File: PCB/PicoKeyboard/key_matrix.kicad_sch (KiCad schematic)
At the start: 170 parts

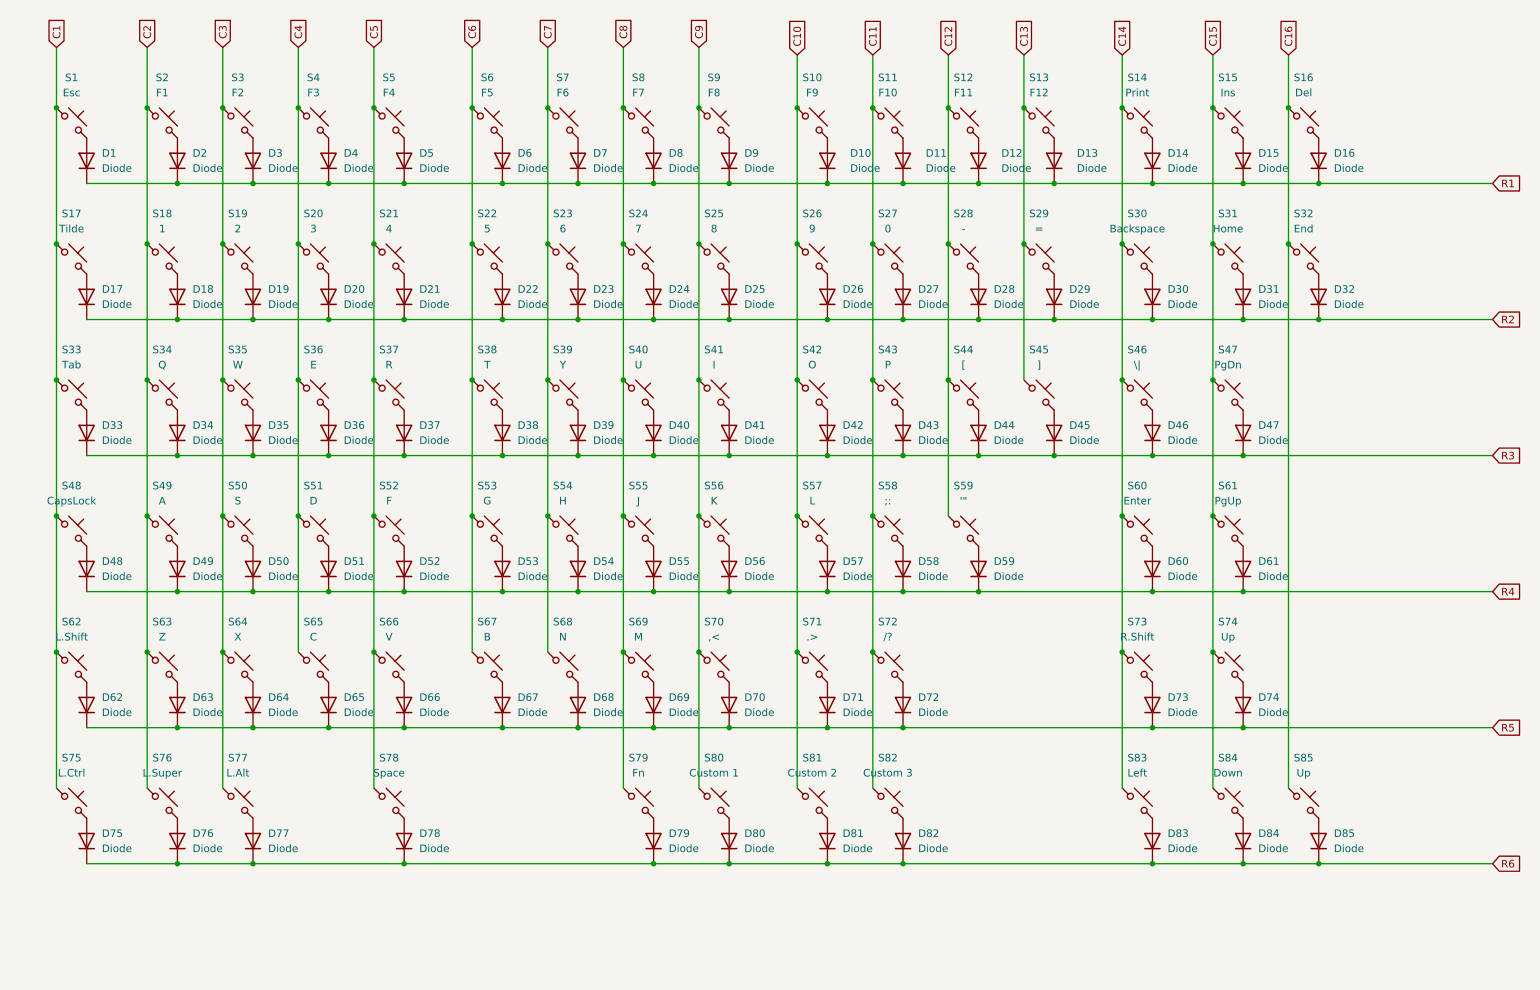
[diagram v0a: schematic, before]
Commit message: New layout
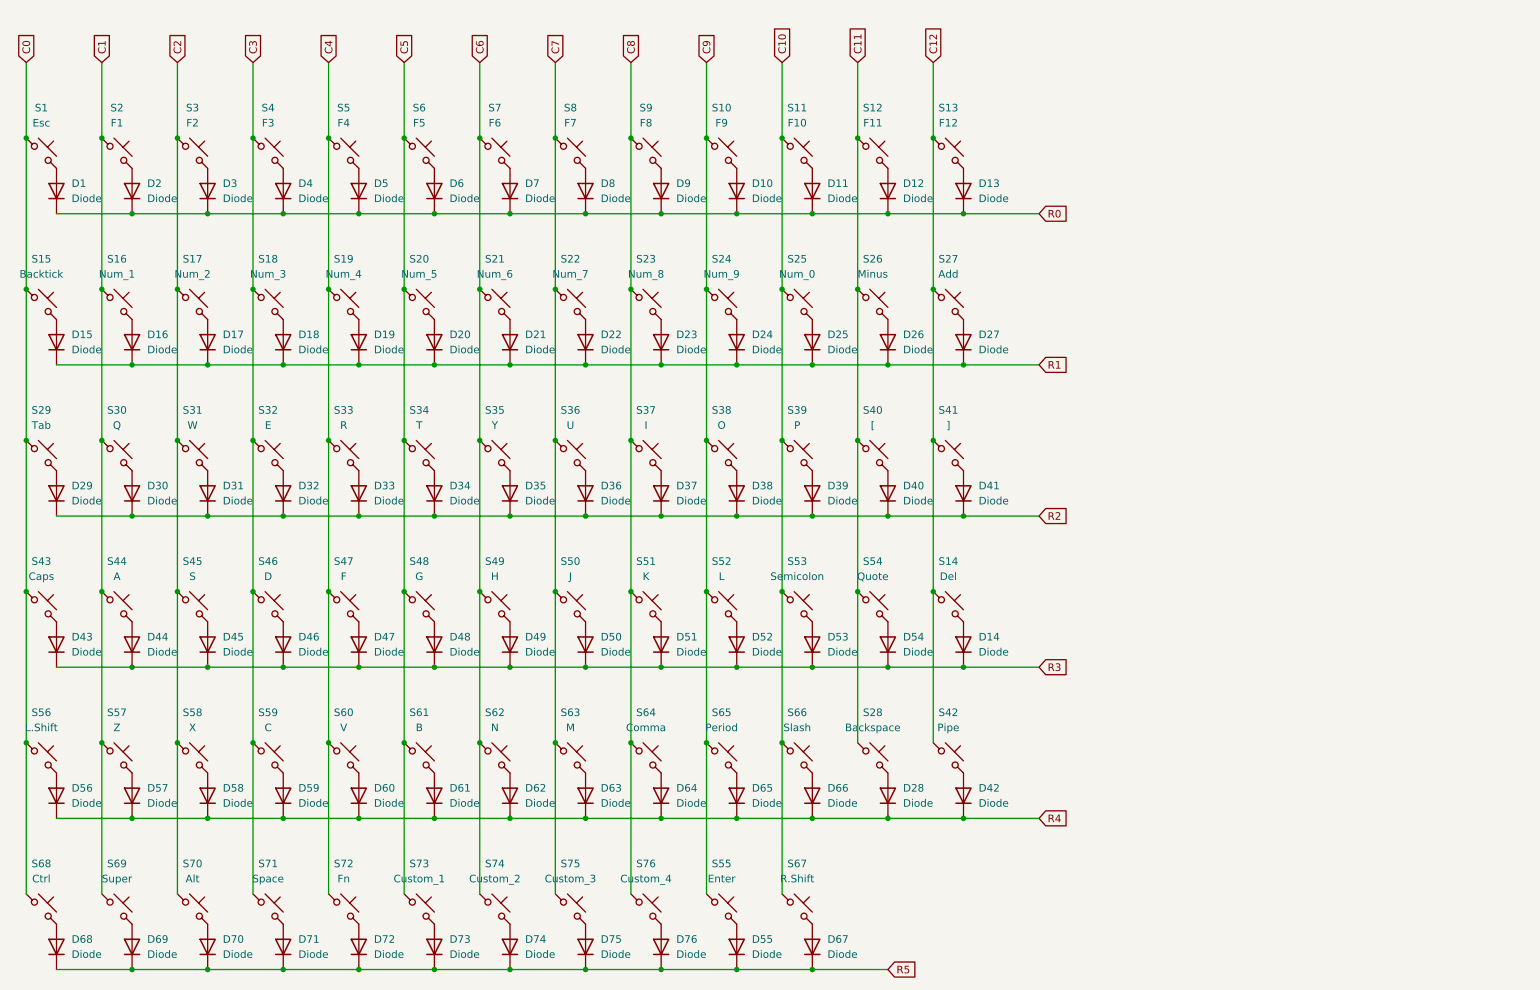
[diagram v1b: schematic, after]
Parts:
- removed D77, D78, D79, D80, D81, D82, D83, D84, D85: Diode, ScottoKeebs_Components:Diode_SOD-123, symbol ScottoKeebs:Placeholder_Diode
- removed S77: L.Alt, Button_Switch_Keyboard:SW_Cherry_MX_1.25u_PCB, symbol ScottoKeebs:Placeholder_Keyswitch
- removed S78: Space, Button_Switch_Keyboard:SW_Cherry_MX_6.25u_PCB, symbol ScottoKeebs:Placeholder_Keyswitch
- removed S79: Fn, Button_Switch_Keyboard:SW_Cherry_MX_1.00u_PCB, symbol ScottoKeebs:Placeholder_Keyswitch
- removed S80: Custom 1, Button_Switch_Keyboard:SW_Cherry_MX_1.00u_PCB, symbol ScottoKeebs:Placeholder_Keyswitch
- removed S81: Custom 2, Button_Switch_Keyboard:SW_Cherry_MX_1.00u_PCB, symbol ScottoKeebs:Placeholder_Keyswitch
- removed S82: Custom 3, Button_Switch_Keyboard:SW_Cherry_MX_1.00u_PCB, symbol ScottoKeebs:Placeholder_Keyswitch
- removed S83: Left, Button_Switch_Keyboard:SW_Cherry_MX_1.00u_PCB, symbol ScottoKeebs:Placeholder_Keyswitch
- removed S84: Down, Button_Switch_Keyboard:SW_Cherry_MX_1.00u_PCB, symbol ScottoKeebs:Placeholder_Keyswitch
- removed S85: Up, Button_Switch_Keyboard:SW_Cherry_MX_1.00u_PCB, symbol ScottoKeebs:Placeholder_Keyswitch
- S1, S10, S11, S12, S13, S2, S3, S4, S5, S6, S7, S8, S9: footprint Button_Switch_Keyboard:SW_Cherry_MX_1.00u_PCB -> ScottoKeebs_MX:MX_PCB_1.00u
- S14: value Print -> Del; footprint Button_Switch_Keyboard:SW_Cherry_MX_1.00u_PCB -> ScottoKeebs_MX:MX_PCB_1.00u
- S15: value Ins -> Backtick; footprint Button_Switch_Keyboard:SW_Cherry_MX_1.00u_PCB -> ScottoKeebs_MX:MX_PCB_1.00u
- S16: value Del -> Num_1; footprint Button_Switch_Keyboard:SW_Cherry_MX_1.00u_PCB -> ScottoKeebs_MX:MX_PCB_1.00u
- S17: value Tilde -> Num_2; footprint Button_Switch_Keyboard:SW_Cherry_MX_1.00u_PCB -> ScottoKeebs_MX:MX_PCB_1.00u
- S18: value 1 -> Num_3; footprint Button_Switch_Keyboard:SW_Cherry_MX_1.00u_PCB -> ScottoKeebs_MX:MX_PCB_1.00u
- S19: value 2 -> Num_4; footprint Button_Switch_Keyboard:SW_Cherry_MX_1.00u_PCB -> ScottoKeebs_MX:MX_PCB_1.00u
- S20: value 3 -> Num_5; footprint Button_Switch_Keyboard:SW_Cherry_MX_1.00u_PCB -> ScottoKeebs_MX:MX_PCB_1.00u
- S21: value 4 -> Num_6; footprint Button_Switch_Keyboard:SW_Cherry_MX_1.00u_PCB -> ScottoKeebs_MX:MX_PCB_1.00u
- S22: value 5 -> Num_7; footprint Button_Switch_Keyboard:SW_Cherry_MX_1.00u_PCB -> ScottoKeebs_MX:MX_PCB_1.00u
- S23: value 6 -> Num_8; footprint Button_Switch_Keyboard:SW_Cherry_MX_1.00u_PCB -> ScottoKeebs_MX:MX_PCB_1.00u
- S24: value 7 -> Num_9; footprint Button_Switch_Keyboard:SW_Cherry_MX_1.00u_PCB -> ScottoKeebs_MX:MX_PCB_1.00u
- S25: value 8 -> Num_0; footprint Button_Switch_Keyboard:SW_Cherry_MX_1.00u_PCB -> ScottoKeebs_MX:MX_PCB_1.00u
- S26: value 9 -> Minus; footprint Button_Switch_Keyboard:SW_Cherry_MX_1.00u_PCB -> ScottoKeebs_MX:MX_PCB_1.00u
- S27: value 0 -> Add; footprint Button_Switch_Keyboard:SW_Cherry_MX_1.00u_PCB -> ScottoKeebs_MX:MX_PCB_1.00u
- S28: value - -> Backspace; footprint Button_Switch_Keyboard:SW_Cherry_MX_1.00u_PCB -> ScottoKeebs_MX:MX_PCB_2.00u
- S29: value = -> Tab; footprint Button_Switch_Keyboard:SW_Cherry_MX_1.00u_PCB -> ScottoKeebs_MX:MX_PCB_1.50u
- S30: value Backspace -> Q; footprint Button_Switch_Keyboard:SW_Cherry_MX_2.00u_PCB -> ScottoKeebs_MX:MX_PCB_1.00u
- S31: value Home -> W; footprint Button_Switch_Keyboard:SW_Cherry_MX_1.00u_PCB -> ScottoKeebs_MX:MX_PCB_1.00u
- S32: value End -> E; footprint Button_Switch_Keyboard:SW_Cherry_MX_1.00u_PCB -> ScottoKeebs_MX:MX_PCB_1.00u
- S33: value Tab -> R; footprint Button_Switch_Keyboard:SW_Cherry_MX_1.50u_PCB -> ScottoKeebs_MX:MX_PCB_1.00u
- S34: value Q -> T; footprint Button_Switch_Keyboard:SW_Cherry_MX_1.00u_PCB -> ScottoKeebs_MX:MX_PCB_1.00u
- S35: value W -> Y; footprint Button_Switch_Keyboard:SW_Cherry_MX_1.00u_PCB -> ScottoKeebs_MX:MX_PCB_1.00u
- S36: value E -> U; footprint Button_Switch_Keyboard:SW_Cherry_MX_1.00u_PCB -> ScottoKeebs_MX:MX_PCB_1.00u
- S37: value R -> I; footprint Button_Switch_Keyboard:SW_Cherry_MX_1.00u_PCB -> ScottoKeebs_MX:MX_PCB_1.00u
- S38: value T -> O; footprint Button_Switch_Keyboard:SW_Cherry_MX_1.00u_PCB -> ScottoKeebs_MX:MX_PCB_1.00u
- S39: value Y -> P; footprint Button_Switch_Keyboard:SW_Cherry_MX_1.00u_PCB -> ScottoKeebs_MX:MX_PCB_1.00u
- S40: value U -> [; footprint Button_Switch_Keyboard:SW_Cherry_MX_1.00u_PCB -> ScottoKeebs_MX:MX_PCB_1.00u
- S41: value I -> ]; footprint Button_Switch_Keyboard:SW_Cherry_MX_1.00u_PCB -> ScottoKeebs_MX:MX_PCB_1.00u
- S42: value O -> Pipe; footprint Button_Switch_Keyboard:SW_Cherry_MX_1.00u_PCB -> ScottoKeebs_MX:MX_PCB_1.50u
- S43: value P -> Caps; footprint Button_Switch_Keyboard:SW_Cherry_MX_1.00u_PCB -> ScottoKeebs_MX:MX_PCB_1.75u
- S44: value [ -> A; footprint Button_Switch_Keyboard:SW_Cherry_MX_1.00u_PCB -> ScottoKeebs_MX:MX_PCB_1.00u
- S45: value ] -> S; footprint Button_Switch_Keyboard:SW_Cherry_MX_1.00u_PCB -> ScottoKeebs_MX:MX_PCB_1.00u
- S46: value \| -> D; footprint Button_Switch_Keyboard:SW_Cherry_MX_1.50u_PCB -> ScottoKeebs_MX:MX_PCB_1.00u
- S47: value PgDn -> F; footprint Button_Switch_Keyboard:SW_Cherry_MX_1.00u_PCB -> ScottoKeebs_MX:MX_PCB_1.00u
- S48: value CapsLock -> G; footprint Button_Switch_Keyboard:SW_Cherry_MX_1.75u_PCB -> ScottoKeebs_MX:MX_PCB_1.00u
- S49: value A -> H; footprint Button_Switch_Keyboard:SW_Cherry_MX_1.00u_PCB -> ScottoKeebs_MX:MX_PCB_1.00u
- S50: value S -> J; footprint Button_Switch_Keyboard:SW_Cherry_MX_1.00u_PCB -> ScottoKeebs_MX:MX_PCB_1.00u
- S51: value D -> K; footprint Button_Switch_Keyboard:SW_Cherry_MX_1.00u_PCB -> ScottoKeebs_MX:MX_PCB_1.00u
- S52: value F -> L; footprint Button_Switch_Keyboard:SW_Cherry_MX_1.00u_PCB -> ScottoKeebs_MX:MX_PCB_1.00u
- S53: value G -> Semicolon; footprint Button_Switch_Keyboard:SW_Cherry_MX_1.00u_PCB -> ScottoKeebs_MX:MX_PCB_1.00u
- S54: value H -> Quote; footprint Button_Switch_Keyboard:SW_Cherry_MX_1.00u_PCB -> ScottoKeebs_MX:MX_PCB_1.00u
- S55: value J -> Enter; footprint Button_Switch_Keyboard:SW_Cherry_MX_1.00u_PCB -> ScottoKeebs_MX:MX_PCB_2.25u
- S56: value K -> L.Shift; footprint Button_Switch_Keyboard:SW_Cherry_MX_1.00u_PCB -> ScottoKeebs_MX:MX_PCB_2.25u
- S57: value L -> Z; footprint Button_Switch_Keyboard:SW_Cherry_MX_1.00u_PCB -> ScottoKeebs_MX:MX_PCB_1.00u
- S58: value ;: -> X; footprint Button_Switch_Keyboard:SW_Cherry_MX_1.00u_PCB -> ScottoKeebs_MX:MX_PCB_1.00u
- S59: value '" -> C; footprint Button_Switch_Keyboard:SW_Cherry_MX_1.00u_PCB -> ScottoKeebs_MX:MX_PCB_1.00u
- S60: value Enter -> V; footprint Button_Switch_Keyboard:SW_Cherry_MX_2.25u_PCB -> ScottoKeebs_MX:MX_PCB_1.00u
- S61: value PgUp -> B; footprint Button_Switch_Keyboard:SW_Cherry_MX_1.00u_PCB -> ScottoKeebs_MX:MX_PCB_1.00u
- S62: value L.Shift -> N; footprint Button_Switch_Keyboard:SW_Cherry_MX_2.25u_PCB -> ScottoKeebs_MX:MX_PCB_1.00u
- S63: value Z -> M; footprint Button_Switch_Keyboard:SW_Cherry_MX_1.00u_PCB -> ScottoKeebs_MX:MX_PCB_1.00u
- S64: value X -> Comma; footprint Button_Switch_Keyboard:SW_Cherry_MX_1.00u_PCB -> ScottoKeebs_MX:MX_PCB_1.00u
- S65: value C -> Period; footprint Button_Switch_Keyboard:SW_Cherry_MX_1.00u_PCB -> ScottoKeebs_MX:MX_PCB_1.00u
- S66: value V -> Slash; footprint Button_Switch_Keyboard:SW_Cherry_MX_1.00u_PCB -> ScottoKeebs_MX:MX_PCB_1.00u
- S67: value B -> R.Shift; footprint Button_Switch_Keyboard:SW_Cherry_MX_1.00u_PCB -> ScottoKeebs_MX:MX_PCB_2.75u
- S68: value N -> Ctrl; footprint Button_Switch_Keyboard:SW_Cherry_MX_1.00u_PCB -> ScottoKeebs_MX:MX_PCB_1.25u
- S69: value M -> Super; footprint Button_Switch_Keyboard:SW_Cherry_MX_1.00u_PCB -> ScottoKeebs_MX:MX_PCB_1.25u
- S70: value ,< -> Alt; footprint Button_Switch_Keyboard:SW_Cherry_MX_1.00u_PCB -> ScottoKeebs_MX:MX_PCB_1.25u
- S71: value .> -> Space; footprint Button_Switch_Keyboard:SW_Cherry_MX_1.00u_PCB -> ScottoKeebs_MX:MX_PCB_6.25u
- S72: value /? -> Fn; footprint Button_Switch_Keyboard:SW_Cherry_MX_1.00u_PCB -> ScottoKeebs_MX:MX_PCB_1.00u
- S73: value R.Shift -> Custom_1; footprint Button_Switch_Keyboard:SW_Cherry_MX_2.75u_PCB -> ScottoKeebs_MX:MX_PCB_1.00u
- S74: value Up -> Custom_2; footprint Button_Switch_Keyboard:SW_Cherry_MX_1.00u_PCB -> ScottoKeebs_MX:MX_PCB_1.00u
- S75: value L.Ctrl -> Custom_3; footprint Button_Switch_Keyboard:SW_Cherry_MX_1.25u_PCB -> ScottoKeebs_MX:MX_PCB_1.00u
- S76: value L.Super -> Custom_4; footprint Button_Switch_Keyboard:SW_Cherry_MX_1.25u_PCB -> ScottoKeebs_MX:MX_PCB_1.00u
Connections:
- net R6 is gone; now on net R5: D75.1 (K), D76.1 (K)
- net C1: now also S16.1, S2.1, S30.1, S44.1, S57.1, S69.1; no longer S1.1, S17.1, S33.1, S48.1, S62.1, S75.1
- net C10: now also S11.1, S25.1, S39.1, S53.1, S66.1, S67.1; no longer S10.1, S26.1, S42.1, S57.1, S71.1
- net C11: now also S12.1, S26.1, S28.1, S40.1, S54.1; no longer S11.1, S27.1, S43.1, S58.1, S72.1
- net C12: now also S13.1, S14.1, S27.1, S41.1, S42.1; no longer S12.1, S28.1, S44.1, S59.1
- net C2: now also S17.1, S3.1, S31.1, S45.1, S58.1, S70.1; no longer S18.1, S2.1, S34.1, S49.1, S63.1, S76.1
- net C3: now also S18.1, S32.1, S4.1, S46.1, S59.1, S71.1; no longer S19.1, S3.1, S35.1, S50.1, S64.1
- net C4: now also S19.1, S33.1, S47.1, S5.1, S60.1, S72.1; no longer S20.1, S36.1, S4.1, S51.1, S65.1
- net C5: now also S20.1, S34.1, S48.1, S6.1, S61.1, S73.1; no longer S21.1, S37.1, S5.1, S52.1, S66.1
- net C6: now also S21.1, S35.1, S49.1, S62.1, S7.1, S74.1; no longer S22.1, S38.1, S53.1, S6.1, S67.1
- net C7: now also S22.1, S36.1, S50.1, S63.1, S75.1, S8.1; no longer S23.1, S39.1, S54.1, S68.1, S7.1
- net C8: now also S23.1, S37.1, S51.1, S64.1, S76.1, S9.1; no longer S24.1, S40.1, S55.1, S69.1, S8.1
- net C9: now also S10.1, S24.1, S38.1, S52.1, S55.1, S65.1; no longer S25.1, S41.1, S56.1, S70.1, S9.1
- net R1: now also D17.1 (K), D18.1 (K), D19.1 (K), D20.1 (K), D21.1 (K), D22.1 (K), D23.1 (K), D24.1 (K), D25.1 (K), D26.1 (K), D27.1 (K); no longer D1.1 (K), D10.1 (K), D11.1 (K), D12.1 (K), D13.1 (K), D14.1 (K), D2.1 (K), D3.1 (K), D4.1 (K), D5.1 (K), D6.1 (K), D7.1 (K), D8.1 (K), D9.1 (K)
- net R2: now also D33.1 (K), D34.1 (K), D35.1 (K), D36.1 (K), D37.1 (K), D38.1 (K), D39.1 (K), D40.1 (K), D41.1 (K); no longer D17.1 (K), D18.1 (K), D19.1 (K), D20.1 (K), D21.1 (K), D22.1 (K), D23.1 (K), D24.1 (K), D25.1 (K), D26.1 (K), D27.1 (K), D28.1 (K)
- net R3: now also D14.1 (K), D48.1 (K), D49.1 (K), D50.1 (K), D51.1 (K), D52.1 (K), D53.1 (K), D54.1 (K); no longer D33.1 (K), D34.1 (K), D35.1 (K), D36.1 (K), D37.1 (K), D38.1 (K), D39.1 (K), D40.1 (K), D41.1 (K), D42.1 (K)
- net R4: now also D28.1 (K), D42.1 (K), D62.1 (K), D63.1 (K), D64.1 (K), D65.1 (K), D66.1 (K); no longer D48.1 (K), D49.1 (K), D50.1 (K), D51.1 (K), D52.1 (K), D53.1 (K), D54.1 (K), D55.1 (K)
- net R5: now also D55.1 (K); no longer D62.1 (K), D63.1 (K), D64.1 (K), D65.1 (K), D66.1 (K)
- removed net C13: S13.1, S29.1, S45.1
- removed net C14: S14.1, S30.1, S46.1, S60.1, S73.1
- removed net C15: S15.1, S31.1, S47.1, S61.1, S74.1
- removed net C16: S16.1, S32.1
- new net C0: S1.1, S15.1, S29.1, S43.1, S56.1, S68.1
- new net R0: D1.1 (K), D10.1 (K), D11.1 (K), D12.1 (K), D13.1 (K), D2.1 (K), D3.1 (K), D4.1 (K), D5.1 (K), D6.1 (K), D7.1 (K), D8.1 (K), D9.1 (K)
